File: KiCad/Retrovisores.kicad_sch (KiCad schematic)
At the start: 50 parts, among them J1 Conn_01x02_Pin, J2 Conn_PIC_ICSP_ICD, M1 Motor_DC, M2 Motor_DC, M3 Motor_DC, Q1 AO3400A, Q10 AO3401A, Q11 AO3400A, Q12 AO3401A, Q2 AO3400A, Q3 AO3401A, Q4 AO3401A, Q5 AO3400A, Q6 AO3401A, Q7 AO3400A, Q8 AO3401A, Q9 AO3400A, SW1 SW_SPST, SW10 SW_Push, SW2 SW_SPST, SW3 SW_SPST, SW4 SW_SPST, SW5 SW_SPST, SW6 SW_SPST, SW7 SW_Push, SW8 SW_Push, SW9 SW_Push, U1 PIC32MX250F128D-IPT, U2 SN65HVD232, U3 FT232RL, U4 LT1117-3.3, U5 TSR3-2450N, U6 VL53L1CXV0FY1

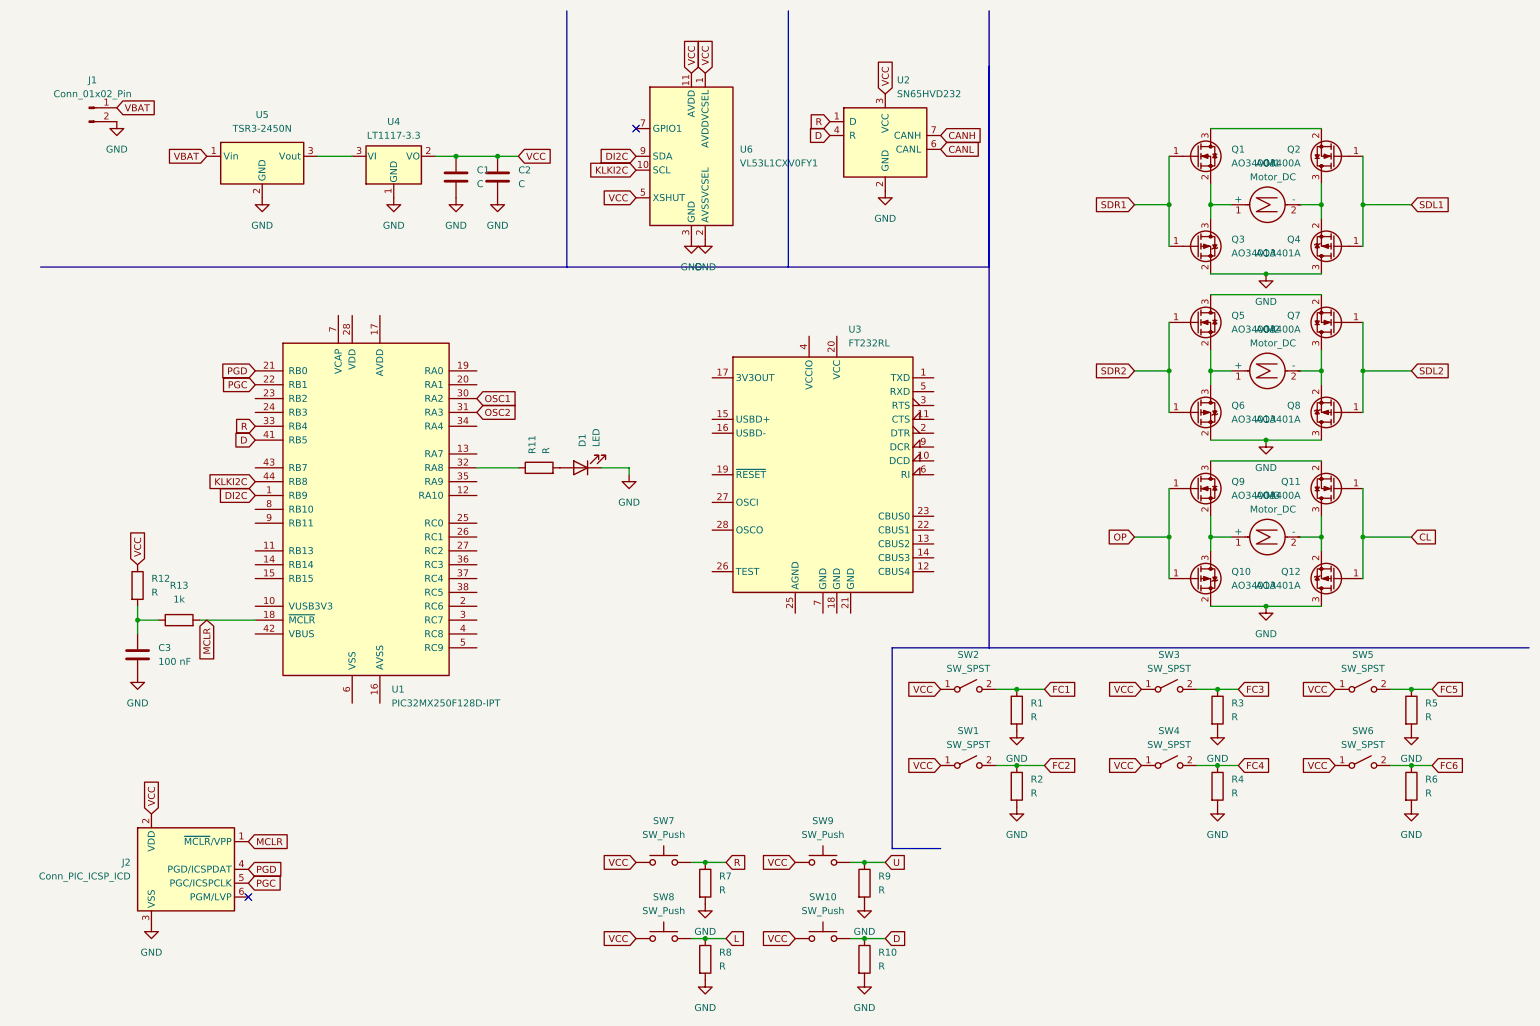
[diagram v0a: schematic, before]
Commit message: he ordenat tot
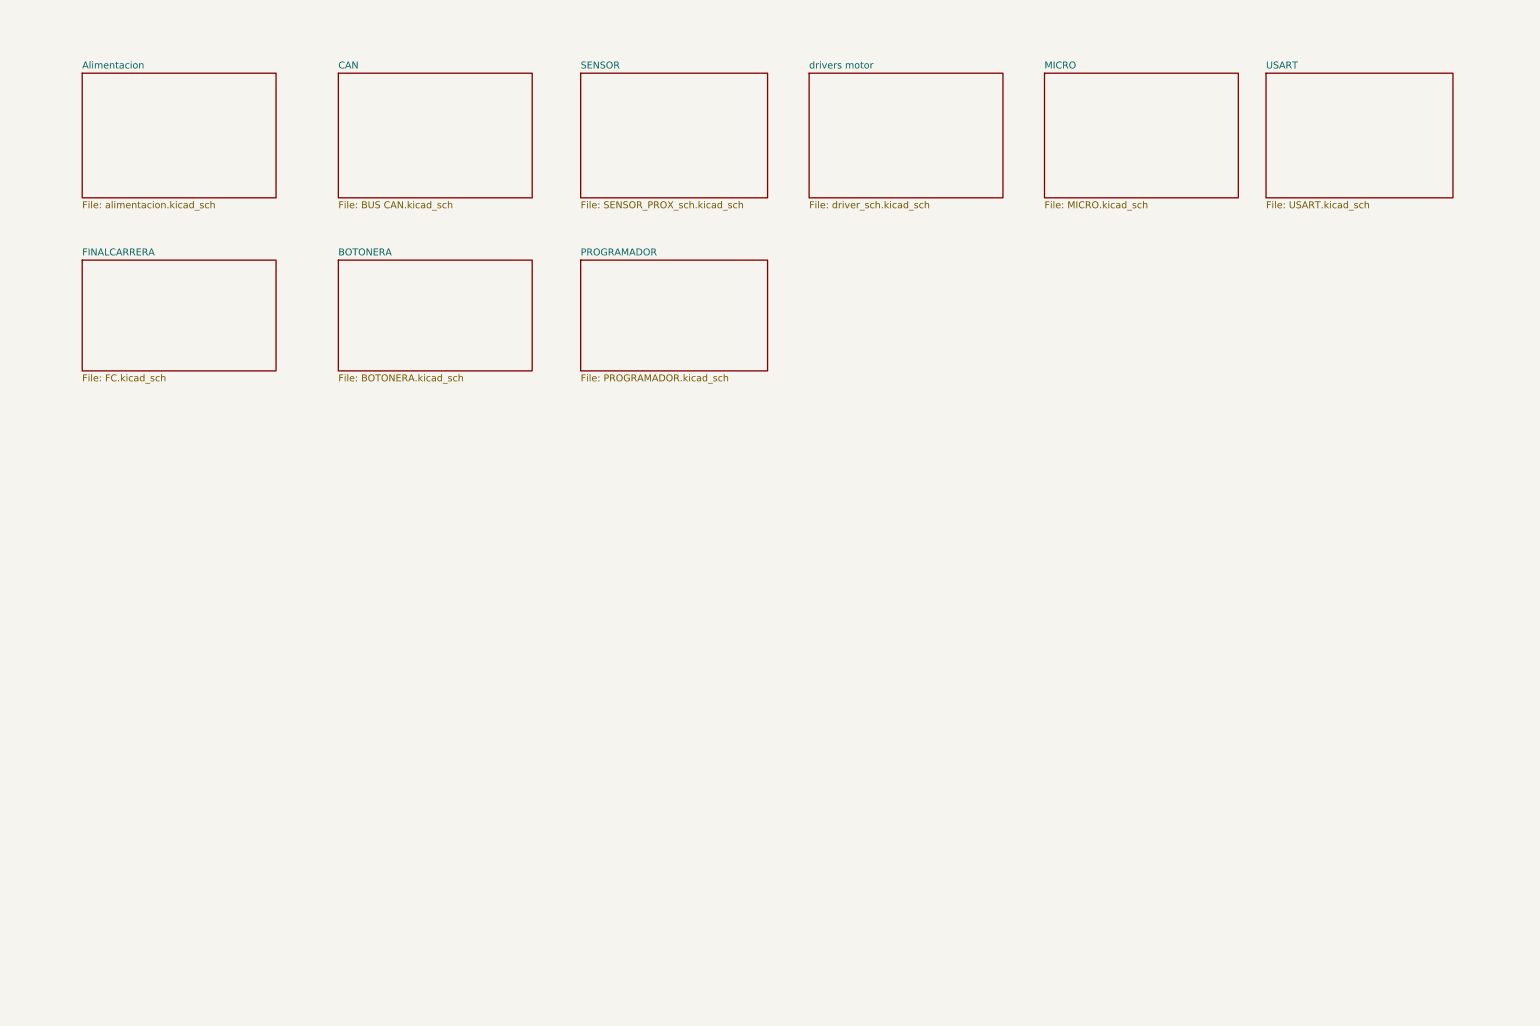
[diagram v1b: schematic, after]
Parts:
- removed C1, C2: C, symbol Device:C
- removed C3: 100 nF, symbol Device:C
- removed D1: LED, symbol Device:LED
- removed J1: Conn_01x02_Pin, symbol Connector:Conn_01x02_Pin
- removed J2: Conn_PIC_ICSP_ICD, symbol Connector:Conn_PIC_ICSP_ICD
- removed M1, M2, M3: Motor_DC, symbol Motor:Motor_DC
- removed Q1, Q11, Q2, Q5, Q7, Q9: AO3400A, Package_TO_SOT_SMD:SOT-23, symbol Transistor_FET:AO3400A
- removed Q10, Q12, Q3, Q4, Q6, Q8: AO3401A, Package_TO_SOT_SMD:SOT-23, symbol Transistor_FET:AO3401A
- removed R1, R10, R11, R12, R2, R3, R4, R5, R6, R7, R8, R9: R, symbol Device:R
- removed R13: 1k, symbol Device:R
- removed SW1, SW2, SW3, SW4, SW5, SW6: SW_SPST, symbol Switch:SW_SPST
- removed SW10, SW7, SW8, SW9: SW_Push, symbol Switch:SW_Push
- removed U1: PIC32MX250F128D-IPT, Package_QFP:TQFP-44_10x10mm_P0.8mm, symbol MCU_Microchip_PIC32:PIC32MX250F128D-IPT
- removed U2: SN65HVD232, Package_SO:SOIC-8_3.9x4.9mm_P1.27mm, symbol Interface_CAN_LIN:SN65HVD232
- removed U3: FT232RL, Package_SO:SSOP-28_5.3x10.2mm_P0.65mm, symbol Interface_USB:FT232RL
- removed U4: LT1117-3.3, symbol Regulator_Linear:LT1117-3.3
- removed U5: TSR3-2450N, Converter_DCDC:Converter_DCDC_TRACO_TSR2-24xxN_TSR2-24xxxN_THT, symbol Converter_DCDC:TSR3-2450N
- removed U6: VL53L1CXV0FY1, Sensor_Distance:ST_VL53L1x, symbol Sensor_Distance:VL53L1CXV0FY1
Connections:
- no-connect marks 2 -> 0
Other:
- added sheet Alimentacion (alimentacion.kicad_sch)
- added sheet BOTONERA (BOTONERA.kicad_sch)
- added sheet CAN (BUS CAN.kicad_sch)
- added sheet FINALCARRERA (FC.kicad_sch)
- added sheet MICRO (MICRO.kicad_sch)
- added sheet PROGRAMADOR (PROGRAMADOR.kicad_sch)
- added sheet SENSOR (SENSOR_PROX_sch.kicad_sch)
- added sheet USART (USART.kicad_sch)
- added sheet drivers motor (driver_sch.kicad_sch)
